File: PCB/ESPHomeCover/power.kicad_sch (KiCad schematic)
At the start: 13 parts, among them J1 24V, U3 AP63203WU-7

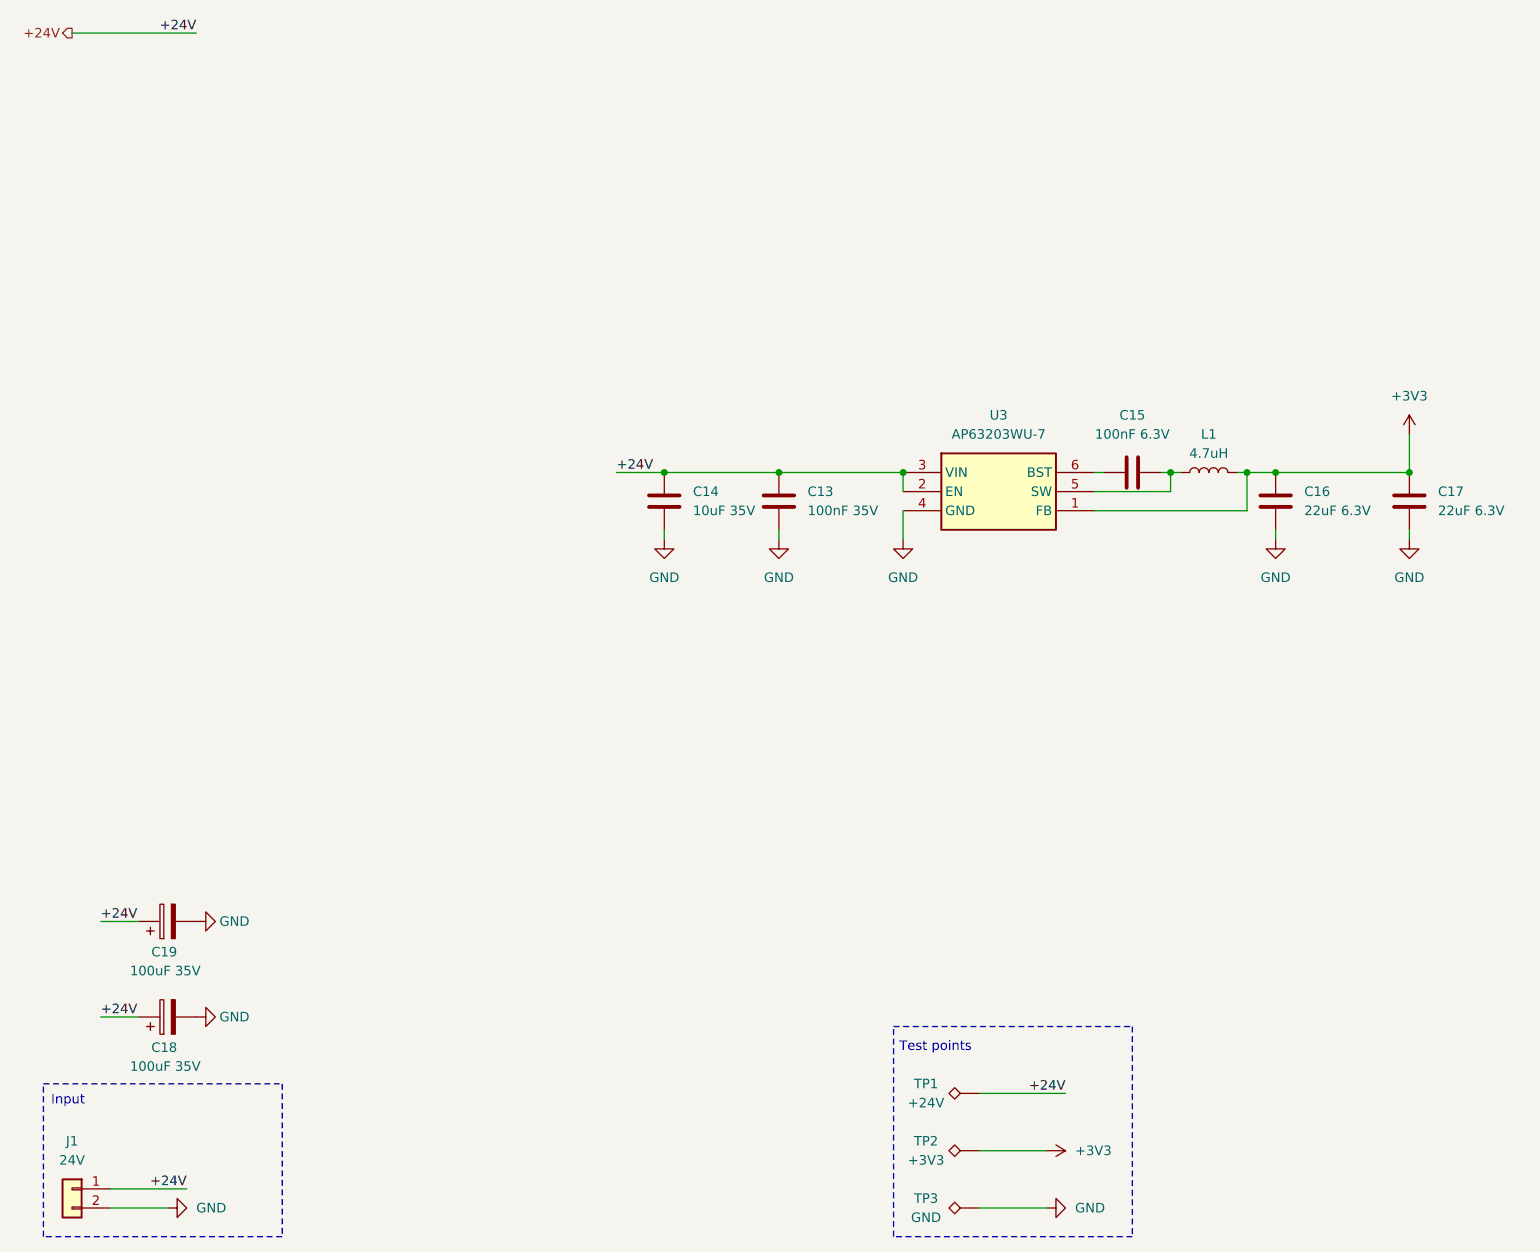
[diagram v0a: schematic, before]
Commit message: update PCB
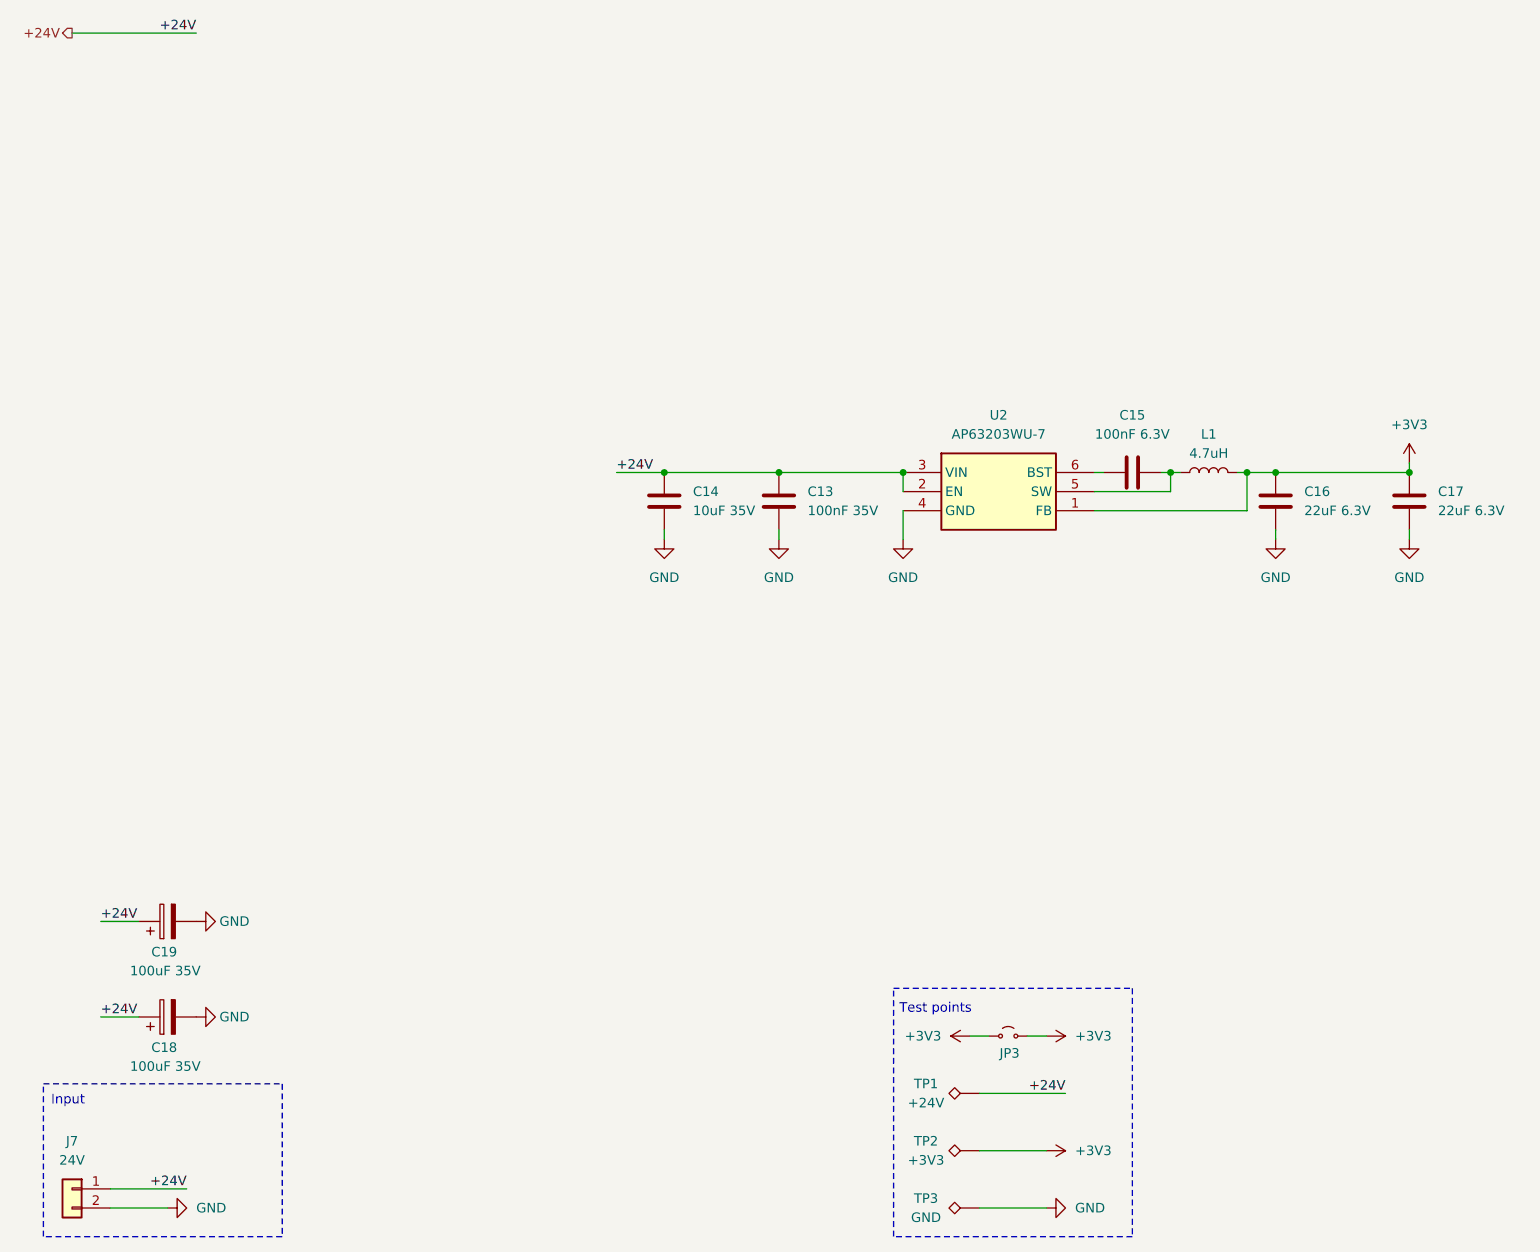
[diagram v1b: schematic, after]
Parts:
- added JP3: ~, Jumper:SolderJumper-2_P1.3mm_Open_RoundedPad1.0x1.5mm, symbol Jumper:Jumper_2_Small_Open
- C13: Mouser Part Number (none) -> 963-GMK107B7104KAHT
- C14: Mouser Part Number (none) -> 81-GRM188R6YA106MA3J
- C15: Mouser Part Number (none) -> 581-06036C104JAT2A
- C16, C17: Mouser Part Number (none) -> 963-MSASJ168BB5226MT
- C18, C19: Mouser Part Number (none) -> 667-EEH-ZK1V101XP
- L1: Mouser Part Number (none) -> 871-B82432T1472K
- renumbered J1 to J7, U3 to U2
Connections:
- net +3V3: now also JP3.1 (A), JP3.2 (B)

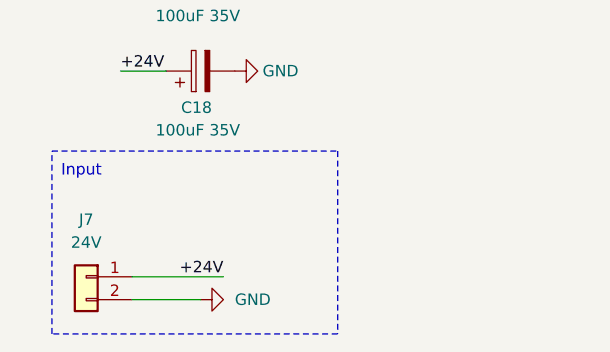
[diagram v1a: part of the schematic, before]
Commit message: update PCB
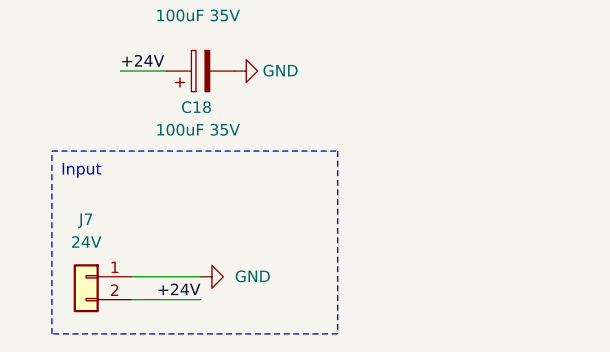
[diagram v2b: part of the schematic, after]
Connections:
- net +24V: now also J7.2 (Pin_2); no longer J7.1 (Pin_1)
- net GND: now also J7.1 (Pin_1); no longer J7.2 (Pin_2)
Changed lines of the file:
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@@
+	(wire
+		(pts
+			(xy 29.21 181.61) (xy 36.83 181.61)
+		)
+		(stroke
+			(width 0)
+			(type default)
+		)
+	)
+	(wire
+		(pts
+			(xy 201.93 85.09) (xy 201.93 86.36)
+		)
+		(stroke
+			(width 0)
+			(type default)
+		)
+	)
+	(wire
+		(pts
+			(xy 160.02 86.36) (xy 161.29 86.36)
+		)
+		(stroke
+			(width 0)
+			(type default)
+		)
+	)
+	(wire
+		(pts
+			(xy 160.02 88.9) (xy 170.18 88.9)
+		)
+		(stroke
+			(width 0)
+			(type default)
+		)
+	)
+	(wire
+		(pts
+			(xy 96.52 86.36) (xy 102.87 86.36)
+		)
+		(stroke
+			(width 0)
+			(type default)
+		)
+	)
+	(wire
+		(pts
+			(xy 180.34 91.44) (xy 180.34 86.36)
+		)
+		(stroke
+			(width 0)
+			(type default)
+		)
+	)
+	(wire
+		(pts
+			(xy 184.15 93.98) (xy 184.15 95.25)
+		)
+		(stroke
+			(width 0)
+			(type default)
+		)
+	)
+	(wire
+		(pts
+			(xy 151.13 161.29) (xy 153.67 161.29)
+		)
+		(stroke
+			(width 0)
+			(type default)
+		)
+	)
 	(wire
 		(pts
 			(xy 29.21 184.15) (xy 36.83 184.15)
-		)
-		(stroke
-			(width 0)
-			(type default)
-		)
-	)
-	(wire
-		(pts
-			(xy 201.93 85.09) (xy 201.93 86.36)
-		)
-		(stroke
-			(width 0)
-			(type default)
-		)
-	)
-	(wire
-		(pts
-			(xy 160.02 86.36) (xy 161.29 86.36)
-		)
-		(stroke
-			(width 0)
-			(type default)
-		)
-	)
-	(wire
-		(pts
-			(xy 160.02 88.9) (xy 170.18 88.9)
-		)
-		(stroke
-			(width 0)
-			(type default)
-		)
-	)
-	(wire
-		(pts
-			(xy 96.52 86.36) (xy 102.87 86.36)
-		)
-		(stroke
-			(width 0)
-			(type default)
-		)
-	)
-	(wire
-		(pts
-			(xy 180.34 91.44) (xy 180.34 86.36)
-		)
-		(stroke
-			(width 0)
-			(type default)
-		)
-	)
-	(wire
-		(pts
-			(xy 184.15 93.98) (xy 184.15 95.25)
-		)
-		(stroke
-			(width 0)
-			(type default)
-		)
-	)
-	(wire
-		(pts
-			(xy 151.13 161.29) (xy 153.67 161.29)
-		)
-		(stroke
-			(width 0)
-			(type default)
-		)
-	)
-	(wire
-		(pts
-			(xy 29.21 181.61) (xy 39.37 181.61)
 		)
 		(stroke
@@
 	)
 	(label "+24V"
-		(at 39.37 181.61 180)
+		(at 36.83 184.15 180)
 		(fields_autoplaced yes)
 		(effects
@@
 	(symbol
 		(lib_id "power:GND")
-		(at 36.83 184.15 90)
+		(at 36.83 181.61 90)
 		(unit 1)
 		(exclude_from_sim no)
@@
 		(fields_autoplaced yes)
 		(property "Reference" "#PWR01"
-			(at 43.18 184.15 0)
+			(at 43.18 181.61 0)
 			(effects
 				(font
@@
 		)
 		(property "Value" "GND"
-			(at 40.64 184.1499 90)
+			(at 40.64 181.6099 90)
 			(effects
 				(font
@@
 		)
 		(property "Footprint" ""
-			(at 36.83 184.15 0)
+			(at 36.83 181.61 0)
 			(effects
 				(font
@@
 		)
 		(property "Datasheet" ""
-			(at 36.83 184.15 0)
+			(at 36.83 181.61 0)
 			(effects
 				(font
@@
 		)
 		(property "Description" "Power symbol creates a global label with name \"GND\" , ground"
-			(at 36.83 184.15 0)
-			(effects
-				(font
+			(at 36.83 181.61 0)
+			(effects
+				(font
